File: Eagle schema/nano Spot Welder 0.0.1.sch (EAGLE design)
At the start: 42 parts, among them Q1 BC548, Q3 BD137, T1 BTA 41 / 600V, U1 NANO, U2 DISPLAY-NOKIA-5110, U3 DS18B20, X3 ~230V, X4 Mikro trafó

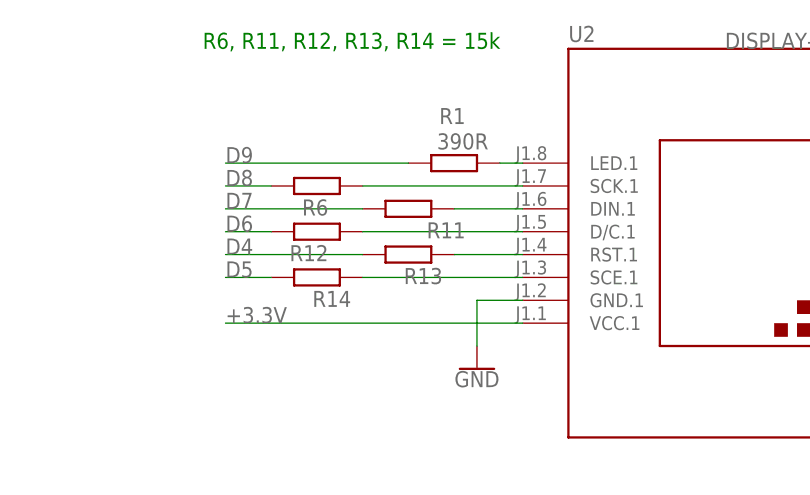
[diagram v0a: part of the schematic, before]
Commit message: - rajzok
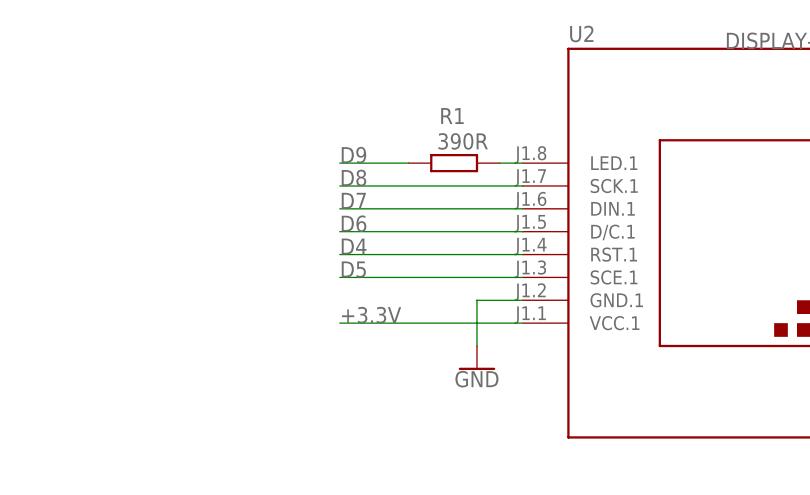
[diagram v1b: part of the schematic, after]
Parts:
- removed R11, R12, R13, R14, R6: (no value), resistor:R-EU_0204/7
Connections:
- removed net N$10: R12.1, U2.D/C.1
- removed net N$11: R13.1, U2.RST.1
- removed net N$12: R14.1, U2.SCE.1
- removed net N$8: R6.1, U2.SCK.1
- removed net N$9: R11.1, U2.DIN.1
- net D4: now also U2.RST.1; no longer R13.2
- net D5: now also U2.SCE.1; no longer R14.2
- net D6: now also U2.D/C.1; no longer R12.2
- net D7: now also U2.DIN.1; no longer R11.2
- net D8: now also U2.SCK.1; no longer R6.2
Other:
- note removed: "R6, R11, R12, R13, R14 = 15k"
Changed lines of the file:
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@@
 <part name="GND9" library="SparkFun-PowerSymbols" library_urn="urn:adsk.eagle:library:530" deviceset="GND" device=""/>
 <part name="R5" library="resistor" library_urn="urn:adsk.eagle:library:348" deviceset="R-EU_" device="0204/7" package3d_urn="urn:adsk.eagle:package:25945/1" value="56kk"/>
-<part name="R6" library="resistor" library_urn="urn:adsk.eagle:library:348" deviceset="R-EU_" device="0204/7" package3d_urn="urn:adsk.eagle:package:25945/1">
-<attribute name="SPICEPREFIX" value="R"/>
-</part>
-<part name="R11" library="resistor" library_urn="urn:adsk.eagle:library:348" deviceset="R-EU_" device="0204/7" package3d_urn="urn:adsk.eagle:package:25945/1"/>
-<part name="R12" library="resistor" library_urn="urn:adsk.eagle:library:348" deviceset="R-EU_" device="0204/7" package3d_urn="urn:adsk.eagle:package:25945/1"/>
-<part name="R13" library="resistor" library_urn="urn:adsk.eagle:library:348" deviceset="R-EU_" device="0204/7" package3d_urn="urn:adsk.eagle:package:25945/1"/>
-<part name="R14" library="resistor" library_urn="urn:adsk.eagle:library:348" deviceset="R-EU_" device="0204/7" package3d_urn="urn:adsk.eagle:package:25945/1"/>
 </parts>
 <sheets>
@@
 <text x="81.28" y="68.58" size="1.778" layer="91">SW</text>
 <text x="81.28" y="66.04" size="1.778" layer="91">DT</text>
-<text x="50.8" y="129.54" size="1.778" layer="91">R6, R11, R12, R13, R14 = 15k</text>
 </plain>
 <instances>
@@
 <attribute name="NAME" x="1.4986" y="-21.59" size="1.778" layer="95" rot="R270"/>
 <attribute name="VALUE" x="-3.302" y="-21.59" size="1.778" layer="96" rot="R270"/>
-</instance>
-<instance part="R6" gate="G$1" x="63.5" y="114.3" smashed="yes" rot="R180">
-<attribute name="NAME" x="64.77" y="112.8014" size="1.778" layer="95" rot="R180"/>
-<attribute name="VALUE" x="67.31" y="117.602" size="1.778" layer="96" rot="R180"/>
-</instance>
-<instance part="R11" gate="G$1" x="73.66" y="111.76" smashed="yes" rot="R180">
-<attribute name="NAME" x="80.01" y="110.2614" size="1.778" layer="95" rot="R180"/>
-<attribute name="VALUE" x="77.47" y="115.062" size="1.778" layer="96" rot="R180"/>
-</instance>
-<instance part="R12" gate="G$1" x="63.5" y="109.22" smashed="yes" rot="R180">
-<attribute name="NAME" x="64.77" y="107.7214" size="1.778" layer="95" rot="R180"/>
-<attribute name="VALUE" x="67.31" y="112.522" size="1.778" layer="96" rot="R180"/>
-</instance>
-<instance part="R13" gate="G$1" x="73.66" y="106.68" smashed="yes" rot="R180">
-<attribute name="NAME" x="77.47" y="105.1814" size="1.778" layer="95" rot="R180"/>
-<attribute name="VALUE" x="77.47" y="109.982" size="1.778" layer="96" rot="R180"/>
-</instance>
-<instance part="R14" gate="G$1" x="63.5" y="104.14" smashed="yes" rot="R180">
-<attribute name="NAME" x="67.31" y="102.6414" size="1.778" layer="95" rot="R180"/>
-<attribute name="VALUE" x="67.31" y="107.442" size="1.778" layer="96" rot="R180"/>
 </instance>
 </instances>
@@
 <segment>
 <pinref part="U2" gate="G$1" pin="VCC.1"/>
-<wire x1="86.36" y1="99.06" x2="53.34" y2="99.06" width="0.1524" layer="91"/>
-<label x="53.34" y="99.06" size="1.778" layer="95"/>
+<wire x1="86.36" y1="99.06" x2="66.04" y2="99.06" width="0.1524" layer="91"/>
+<label x="66.04" y="99.06" size="1.778" layer="95"/>
 </segment>
 <segment>
@@
 <segment>
 <pinref part="R1" gate="G$1" pin="2"/>
-<wire x1="73.66" y1="116.84" x2="53.34" y2="116.84" width="0.1524" layer="91"/>
-<label x="53.34" y="116.84" size="1.778" layer="95"/>
+<wire x1="73.66" y1="116.84" x2="66.04" y2="116.84" width="0.1524" layer="91"/>
+<label x="66.04" y="116.84" size="1.778" layer="95"/>
 </segment>
 <segment>
@@
 </segment>
 <segment>
-<pinref part="R13" gate="G$1" pin="2"/>
-<wire x1="68.58" y1="106.68" x2="53.34" y2="106.68" width="0.1524" layer="91"/>
-<label x="53.34" y="106.68" size="1.778" layer="95"/>
+<wire x1="86.36" y1="106.68" x2="66.04" y2="106.68" width="0.1524" layer="91"/>
+<label x="66.04" y="106.68" size="1.778" layer="95"/>
+<pinref part="U2" gate="G$1" pin="RST.1"/>
 </segment>
 </net>
@@
 </segment>
 <segment>
-<pinref part="R14" gate="G$1" pin="2"/>
-<wire x1="58.42" y1="104.14" x2="53.34" y2="104.14" width="0.1524" layer="91"/>
-<label x="53.34" y="104.14" size="1.778" layer="95"/>
+<label x="66.04" y="104.14" size="1.778" layer="95"/>
+<pinref part="U2" gate="G$1" pin="SCE.1"/>
+<wire x1="86.36" y1="104.14" x2="66.04" y2="104.14" width="0.1524" layer="91"/>
 </segment>
 </net>
@@
 </segment>
 <segment>
-<pinref part="R12" gate="G$1" pin="2"/>
-<wire x1="58.42" y1="109.22" x2="53.34" y2="109.22" width="0.1524" layer="91"/>
-<label x="53.34" y="109.22" size="1.778" layer="95"/>
+<label x="66.04" y="109.22" size="1.778" layer="95"/>
+<pinref part="U2" gate="G$1" pin="D/C.1"/>
+<wire x1="86.36" y1="109.22" x2="66.04" y2="109.22" width="0.1524" layer="91"/>
 </segment>
 </net>
@@
 </segment>
 <segment>
-<pinref part="R11" gate="G$1" pin="2"/>
-<wire x1="68.58" y1="111.76" x2="53.34" y2="111.76" width="0.1524" layer="91"/>
-<label x="53.34" y="111.76" size="1.778" layer="95"/>
+<wire x1="86.36" y1="111.76" x2="66.04" y2="111.76" width="0.1524" layer="91"/>
+<label x="66.04" y="111.76" size="1.778" layer="95"/>
+<pinref part="U2" gate="G$1" pin="DIN.1"/>
 </segment>
 </net>
@@
 </segment>
 <segment>
-<pinref part="R6" gate="G$1" pin="2"/>
-<wire x1="58.42" y1="114.3" x2="53.34" y2="114.3" width="0.1524" layer="91"/>
-<label x="53.34" y="114.3" size="1.778" layer="95"/>
+<label x="66.04" y="114.3" size="1.778" layer="95"/>
+<pinref part="U2" gate="G$1" pin="SCK.1"/>
+<wire x1="86.36" y1="114.3" x2="66.04" y2="114.3" width="0.1524" layer="91"/>
 </segment>
 </net>
@@
 </segment>
 </net>
-<net name="N$8" class="0">
-<segment>
-<pinref part="U2" gate="G$1" pin="SCK.1"/>
-<pinref part="R6" gate="G$1" pin="1"/>
-<wire x1="86.36" y1="114.3" x2="68.58" y2="114.3" width="0.1524" layer="91"/>
-</segment>
-</net>
-<net name="N$9" class="0">
-<segment>
-<pinref part="U2" gate="G$1" pin="DIN.1"/>
-<pinref part="R11" gate="G$1" pin="1"/>
-<wire x1="86.36" y1="111.76" x2="78.74" y2="111.76" width="0.1524" layer="91"/>
-</segment>
-</net>
-<net name="N$10" class="0">
-<segment>
-<pinref part="U2" gate="G$1" pin="D/C.1"/>
-<pinref part="R12" gate="G$1" pin="1"/>
-<wire x1="86.36" y1="109.22" x2="68.58" y2="109.22" width="0.1524" layer="91"/>
-</segment>
-</net>
-<net name="N$11" class="0">
-<segment>
-<pinref part="U2" gate="G$1" pin="RST.1"/>
-<pinref part="R13" gate="G$1" pin="1"/>
-<wire x1="86.36" y1="106.68" x2="78.74" y2="106.68" width="0.1524" layer="91"/>
-</segment>
-</net>
-<net name="N$12" class="0">
-<segment>
-<pinref part="U2" gate="G$1" pin="SCE.1"/>
-<pinref part="R14" gate="G$1" pin="1"/>
-<wire x1="86.36" y1="104.14" x2="68.58" y2="104.14" width="0.1524" layer="91"/>
-</segment>
-</net>
